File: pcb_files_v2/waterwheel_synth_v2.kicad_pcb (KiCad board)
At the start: 2 copper layers, 171.7 x 171.7 mm, 192 parts, among them J1 Drum_SW_BD, J10 LEDS_volca, J11 Drum_Returns, J12 volc audio in/out. button trig, J13 RELAY out, J14 panel pots, J2 Drum_SW_SD, J3 Drum_sw_HH, J4 12x binary outs, 2x ins, J5 LED_drums, J6 Drum_sw_TT, J7 Volca_steps, J8 LED_binary, J9 power and clock, K1 G5Q-1, Q1 2N3904, Q10 2N3904, Q11 2N3904, Q12 2N3904, Q13 2N3904, Q14 2N3904, Q15 2N3904, Q16 2N3904, Q17 2N3904, Q18 2N3904, Q19 2N3904, Q2 2N3904, Q20 2N3904, Q21 2N3904, Q22 2N3904, Q23 2N3904, Q24 2N3904, Q25 2N3904, Q3 2N3904, Q4 2N3904, Q5 2N3904, Q6 2N3904, Q7 2N3904, Q8 2N3904, Q9 2N3904, U1 4017, U10 Teensy3.2, U2 4069, U4 4017, U5 4040, U6 4081, U7 4017, U8 555(NEW_layout), U9 4066

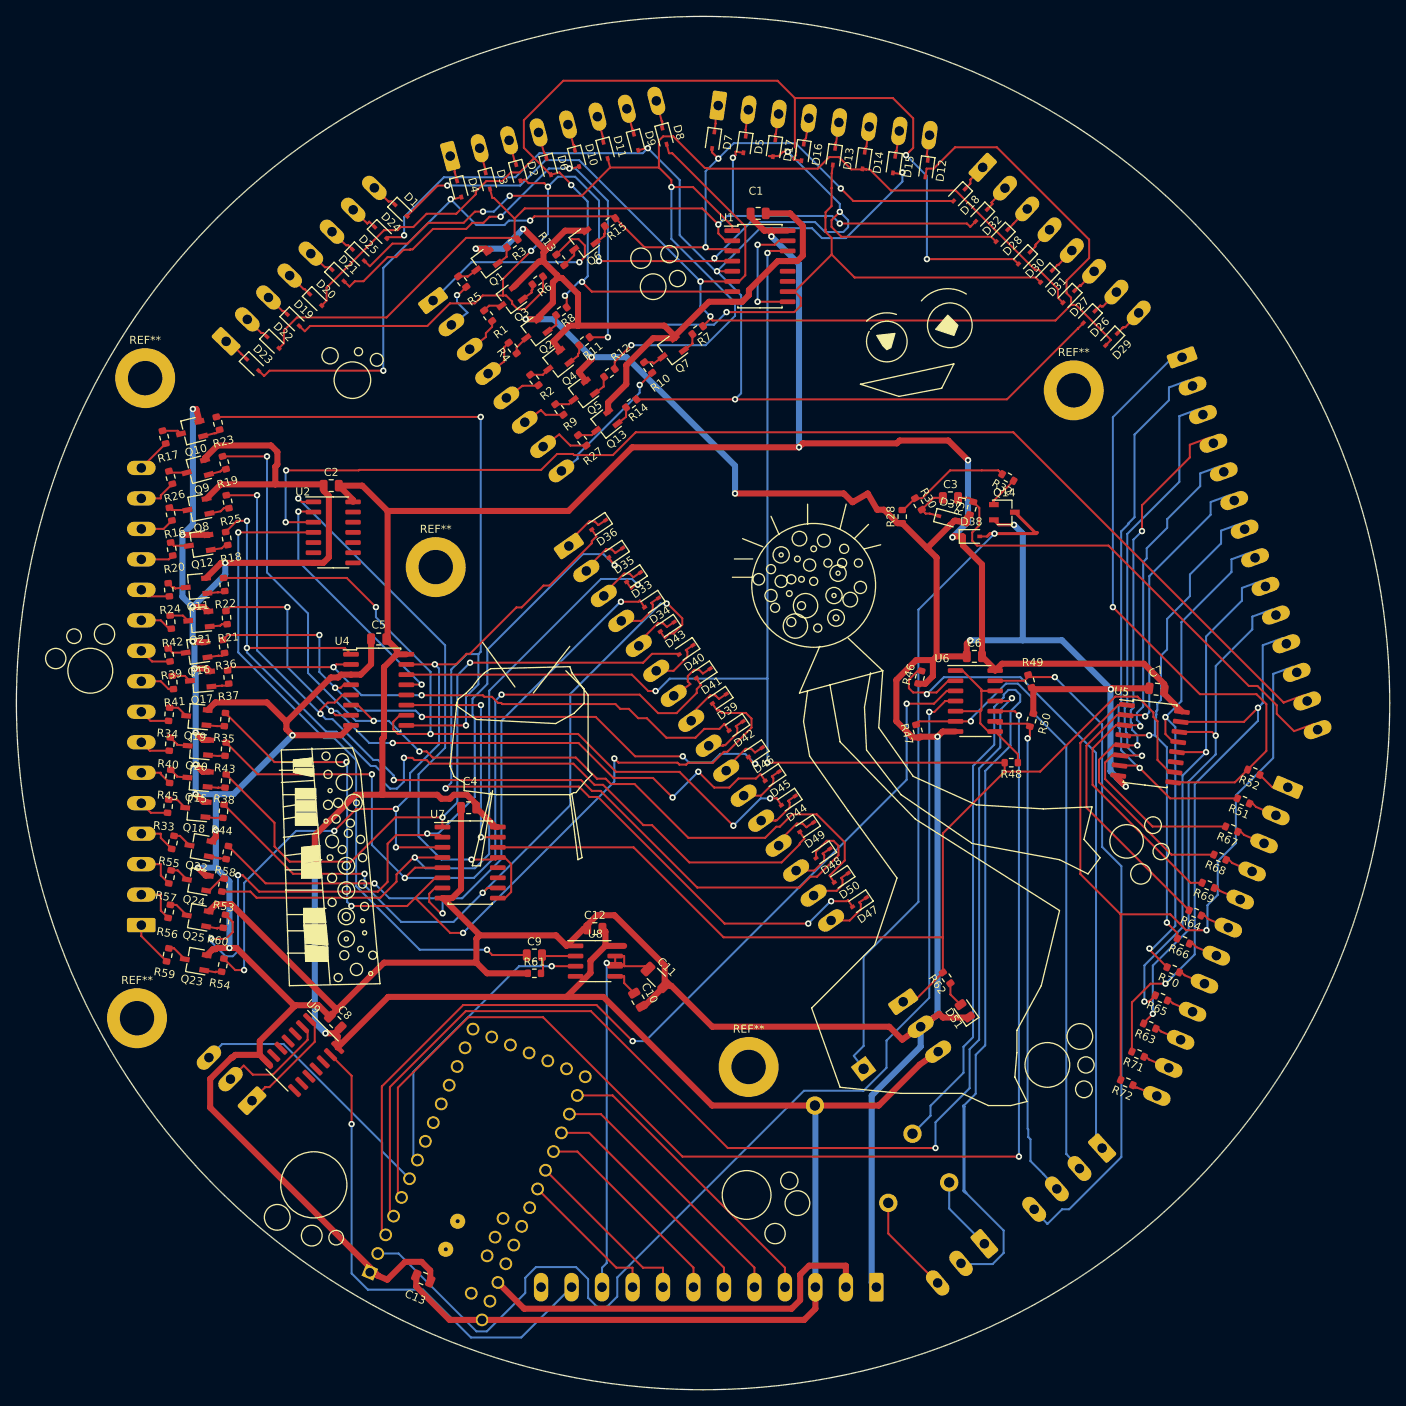
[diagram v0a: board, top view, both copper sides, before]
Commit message: oct 2025 update
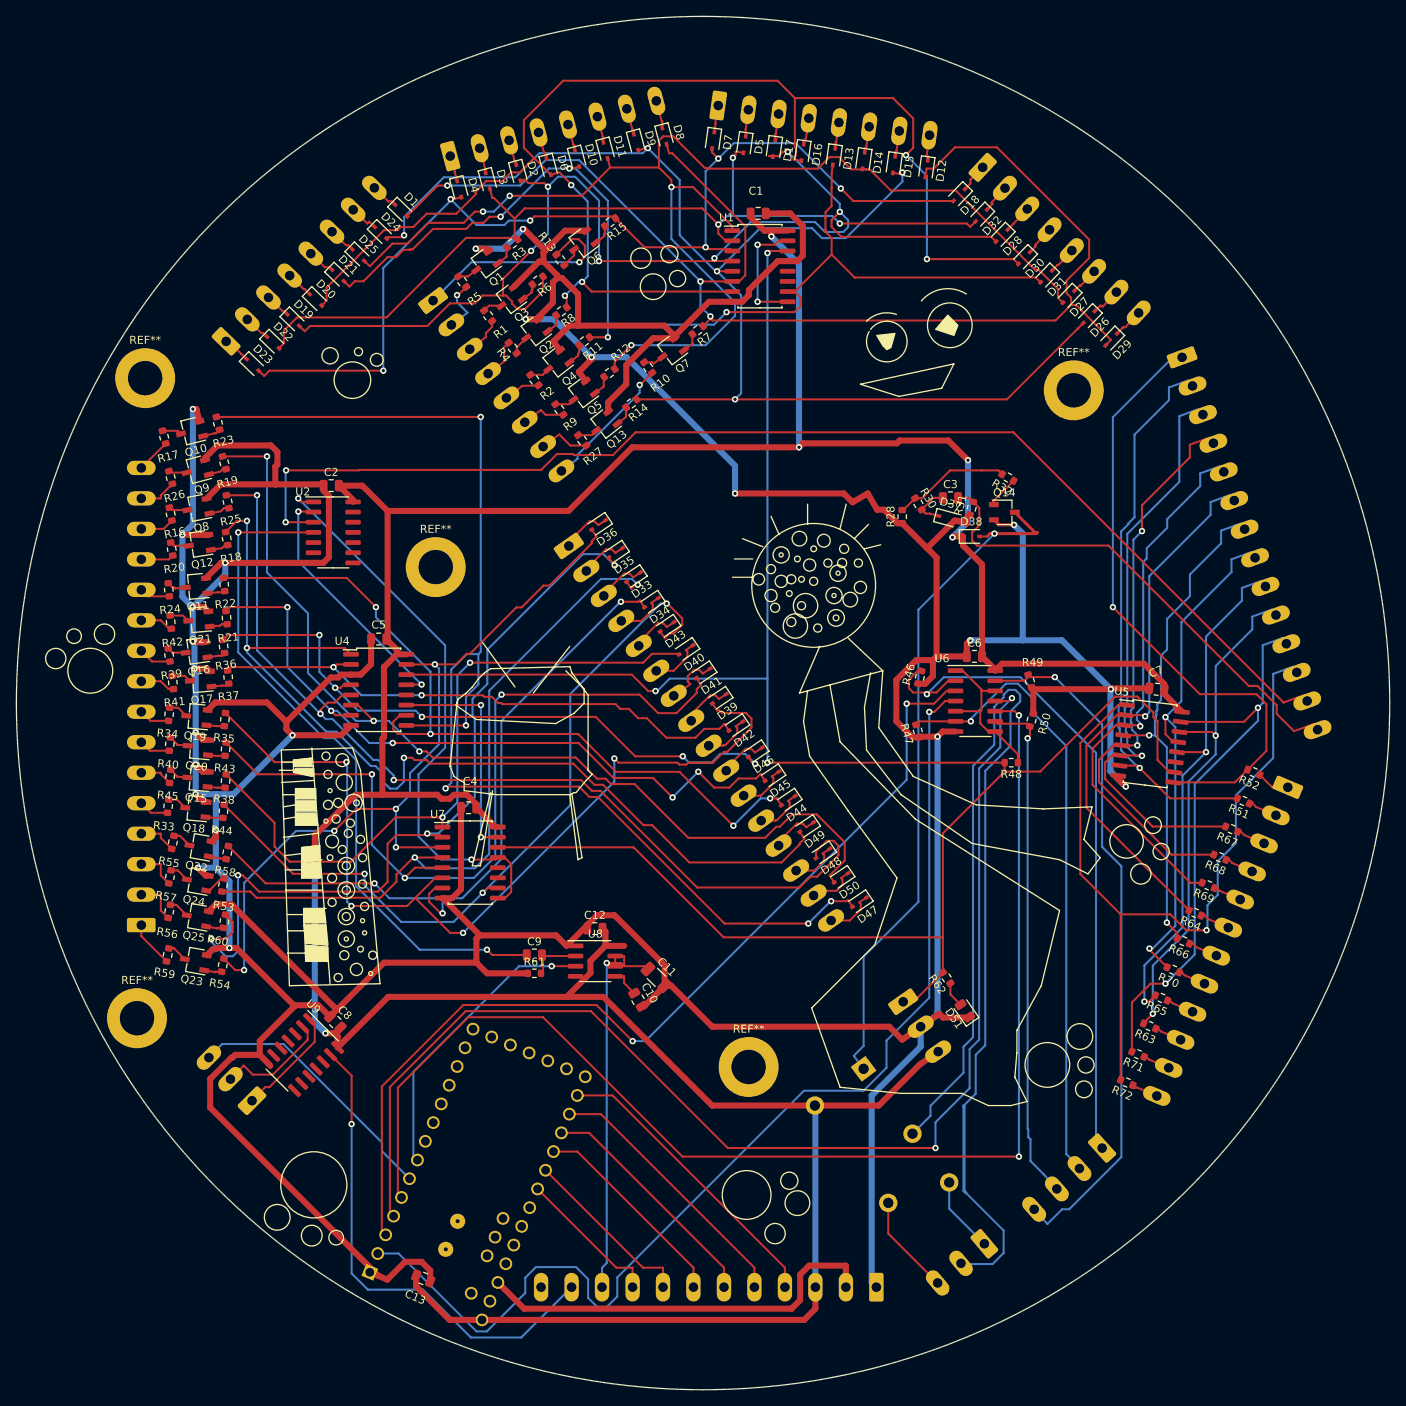
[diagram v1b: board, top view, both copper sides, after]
